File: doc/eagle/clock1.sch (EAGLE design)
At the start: 17 parts, among them J1 LM35, J2 BMP180 sensor, J3 DS1307 RTC, J4 4X3 keypad, J5 DHT11 module, J6 Nokia LCD 5110

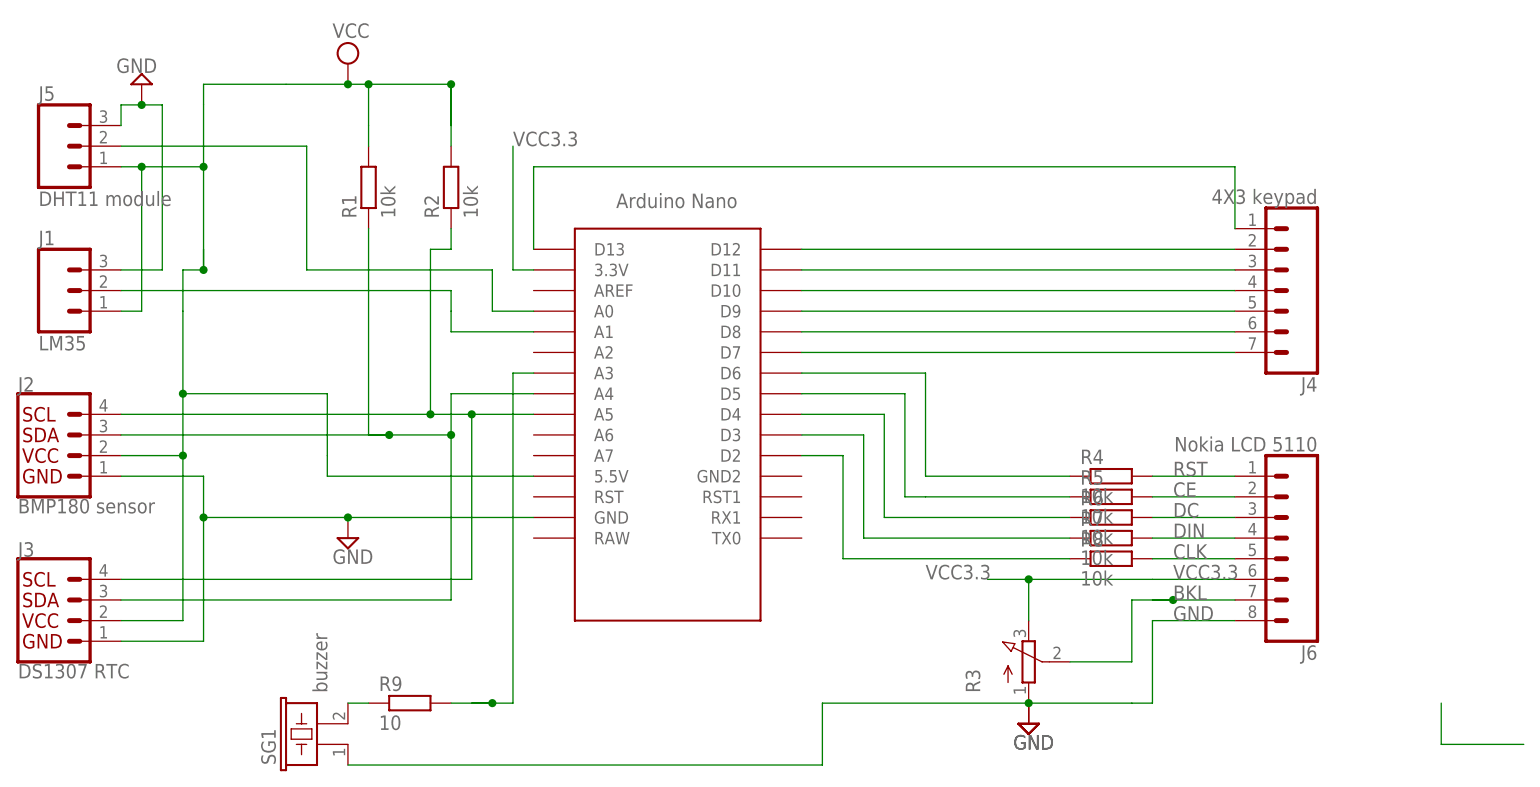
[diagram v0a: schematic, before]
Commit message: Changing sch from fritz to eagle
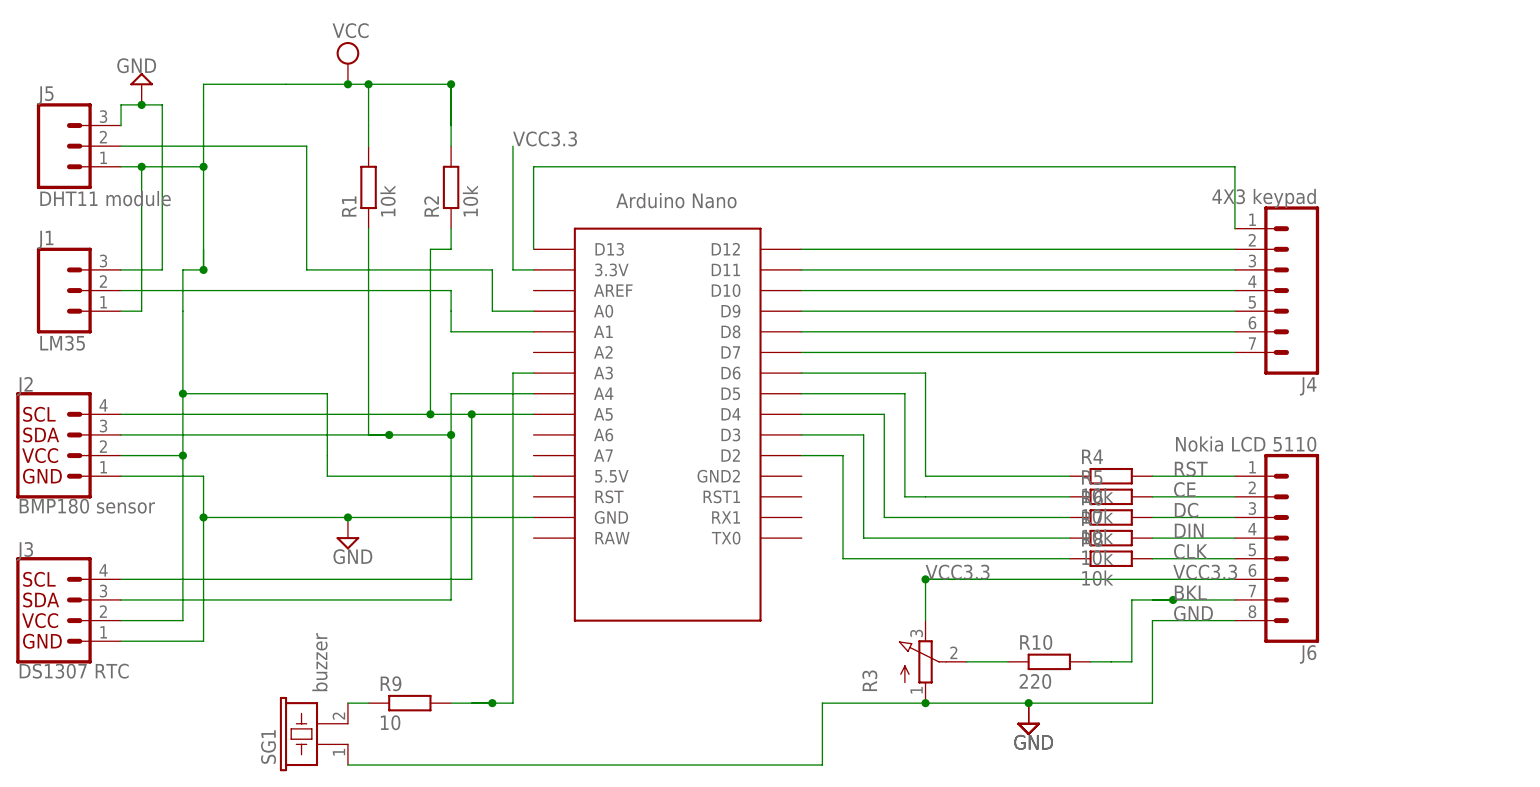
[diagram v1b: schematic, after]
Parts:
- added R10: 220, eagle-ltspice:R0204/7
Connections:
- new net N$20: R10.1, R3.S
- net BKL: now also R10.2; no longer R3.S
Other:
- moved on the sheet: R3
